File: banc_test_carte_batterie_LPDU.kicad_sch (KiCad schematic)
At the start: 1 part, among them J1 DIN41612_3x32

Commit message: version 26/06/2025 08:31
Signed-off-by: TEST-BANC <TEST-BANC@DOMOMICRON.LOCAL>
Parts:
- added J14, J15, J16, J17, J18, J65, J66, J67: Conn_01x0_P2.54mm_pinheader_vertical, Omiconnecteur:PinHeader_1x01_P2.54mm_V_omi, symbol Omiconnecteur:Conn_01x0_P2.54mm_pinheader_vertical
- added J21, J22, J26: Conn_01x04_P2.54mm_pinheader_vertical, Omiconnecteur:PinHeader_1x04_P2.54mm_V_omi, symbol Omiconnecteur:Conn_01x04_P2.54mm_pinheader_vertical
- added J23, J29: Conn_02x08_Odd_Even, Omiconnecteur:PinHeader_2x08_P2.54mm_V_omi, symbol Omiconnecteur:Conn_02x08_Odd_Even_omi
- added J24, J25: Conn_02x08_Odd_Even, Omiconnecteur:PinHeader_2x02_P2.54mm_V_omi, symbol Omiconnecteur:Conn_02x02_Odd_Even_omi
- added R12, R13, R14, R27, R28, R29, R30, R31, R32, R33, R34, R35: 0, symbol Device:R
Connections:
- net GND: now also J1.B10, J1.B11, J1.B12, J1.B5, J1.B6, J1.B7, J1.B8, J1.B9; no longer J1.B1, J1.B2
- net AI7: now reaches J1.A10
- net AO1: now reaches J1.A11
- net AO2: now reaches J1.A12
- net IN0: now reaches J1.A13
- net IN1: now reaches J1.A14
- net IN2: now reaches J1.A15
- net IN3: now reaches J1.A16
- net IN4: now reaches J1.A17
- net IN5: now reaches J1.A18
- net IN6: now reaches J1.A19
- net at J1.A2: now also J67.1 (Pin_1)
- net IN7: now reaches J1.A20
- net at J1.A21: now also J29.2 (Pin_2)
- net at J1.A22: now also J29.4 (Pin_4)
- net at J1.A23: now also J29.6 (Pin_6)
- net at J1.A24: now also J29.8 (Pin_8)
- net at J1.A25: now also J29.10 (Pin_10)
- net at J1.A26: now also J29.12 (Pin_12)
- net at J1.A27: now also J29.14 (Pin_14)
- net at J1.A28: now also J29.16 (Pin_16)
- net at J1.A29: now also J21.1 (Pin_1), R32.1
- net SORTIE_MULTIPLEXEUR: now reaches J1.A3
- net at J1.A30: now also J21.2 (Pin_2), R33.1
- net at J1.A31: now also J21.3 (Pin_3), R34.1
- net at J1.A32: now also J21.4 (Pin_4), R35.1
- net AI1: now reaches J1.A4
- net AI2: now reaches J1.A5
- net AI3: now reaches J1.A6
- net AI4: now reaches J1.A7
- net AI5: now reaches J1.A8
- net AI6: now reaches J1.A9
- net GND_MCP: now reaches J1.B13
- net GND_MCP: now also J1.B14, J1.B15, J1.B16, J1.B17, J1.B18, J1.B19, J1.B20
- net GND_IO_Ana: now reaches J1.B21
- net GND_IO_Ana: now also J1.B22, J1.B23, J1.B24, J1.B25, J1.B26, J1.B27, J1.B28
- net at J1.B29: now also J26.1 (Pin_1), R28.1
- net at J1.B30: now also J26.2 (Pin_2), R29.1
- net at J1.B31: now also J26.3 (Pin_3), R30.1
- net at J1.B32: now also J26.4 (Pin_4), R31.1
- net at J1.C1: now also J65.1 (Pin_1)
- net at J1.C10: now also J23.16 (Pin_16)
- net at J1.C11: now also J14.1 (Pin_1)
- net at J1.C12: now also J15.1 (Pin_1)
- net S1: now reaches J1.C13
- net S2: now reaches J1.C14
- net S3: now reaches J1.C15
- net S4: now reaches J1.C16
- net S5: now reaches J1.C17
- net S6: now reaches J1.C18
- net S7: now reaches J1.C19
- net S7: now also J1.C20
- net at J1.C2: now also J66.1 (Pin_1)
- net COMMOUT: now reaches J1.C21
- net at J1.C22: now also J24.2 (Pin_2)
- net at J1.C23: now also J24.4 (Pin_4)
- net at J1.C24: now also J25.2 (Pin_2)
- net at J1.C25: now also J25.4 (Pin_4)
- net at J1.C26: now also J18.1 (Pin_1)
- net at J1.C27: now also J16.1 (Pin_1)
- net at J1.C28: now also J17.1 (Pin_1)
- net at J1.C29: now also J22.1 (Pin_1), R12.1
- net at J1.C3: now also J23.2 (Pin_2)
- net at J1.C30: now also J22.2 (Pin_2), R13.1
- net at J1.C31: now also J22.3 (Pin_3), R14.1
- net at J1.C32: now also J22.4 (Pin_4), R27.1
- net at J1.C4: now also J23.4 (Pin_4)
- net at J1.C5: now also J23.6 (Pin_6)
- net at J1.C6: now also J23.8 (Pin_8)
- net at J1.C7: now also J23.10 (Pin_10)
- net at J1.C8: now also J23.12 (Pin_12)
- net at J1.C9: now also J23.14 (Pin_14)
- new net +5V_PIC: R28.2
- new net CLK: J25.1 (Pin_1)
- new net GND_ALIM: J1.B1, J1.B2
- new net GND_TS3A: R12.2, R13.2, R14.2, R27.2
- new net I0: J23.1 (Pin_1)
- new net I1: J23.3 (Pin_3)
- new net I2: J23.5 (Pin_5)
- new net I3: J23.7 (Pin_7)
- new net I4: J23.9 (Pin_9)
- new net I5: J23.11 (Pin_11)
- new net I6: J23.13 (Pin_13)
- new net I7: J23.15 (Pin_15)
- new net IO0: J29.1 (Pin_1)
- new net IO1: J29.3 (Pin_3)
- new net IO2: J29.5 (Pin_5)
- new net IO3: J29.7 (Pin_7)
- new net IO4: J29.9 (Pin_9)
- new net IO5: J29.11 (Pin_11)
- new net IO6: J29.13 (Pin_13)
- new net IO7: J29.15 (Pin_15)
- new net PS13: R29.2
- new net PS14: R30.2
- new net PS15: R31.2
- new net Prog_+5V_PIC: R32.2
- new net Prog_PS13: R33.2
- new net Prog_PS14: R34.2
- new net Prog_PS15: R35.2
- new net Rx: J24.3 (Pin_3)
- new net SDA: J25.3 (Pin_3)
- new net Tx: J24.1 (Pin_1)
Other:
- added sheet MCP23017 (MCP23017.kicad_sch)
- added sheet Relais (Relais.kicad_sch)
- added sheet Support pile (Pile.kicad_sch)
- note added: "permetre de connceter une carte relais de 4 si on soude pas la resistance 0 ohm"
- moved on the sheet: J1

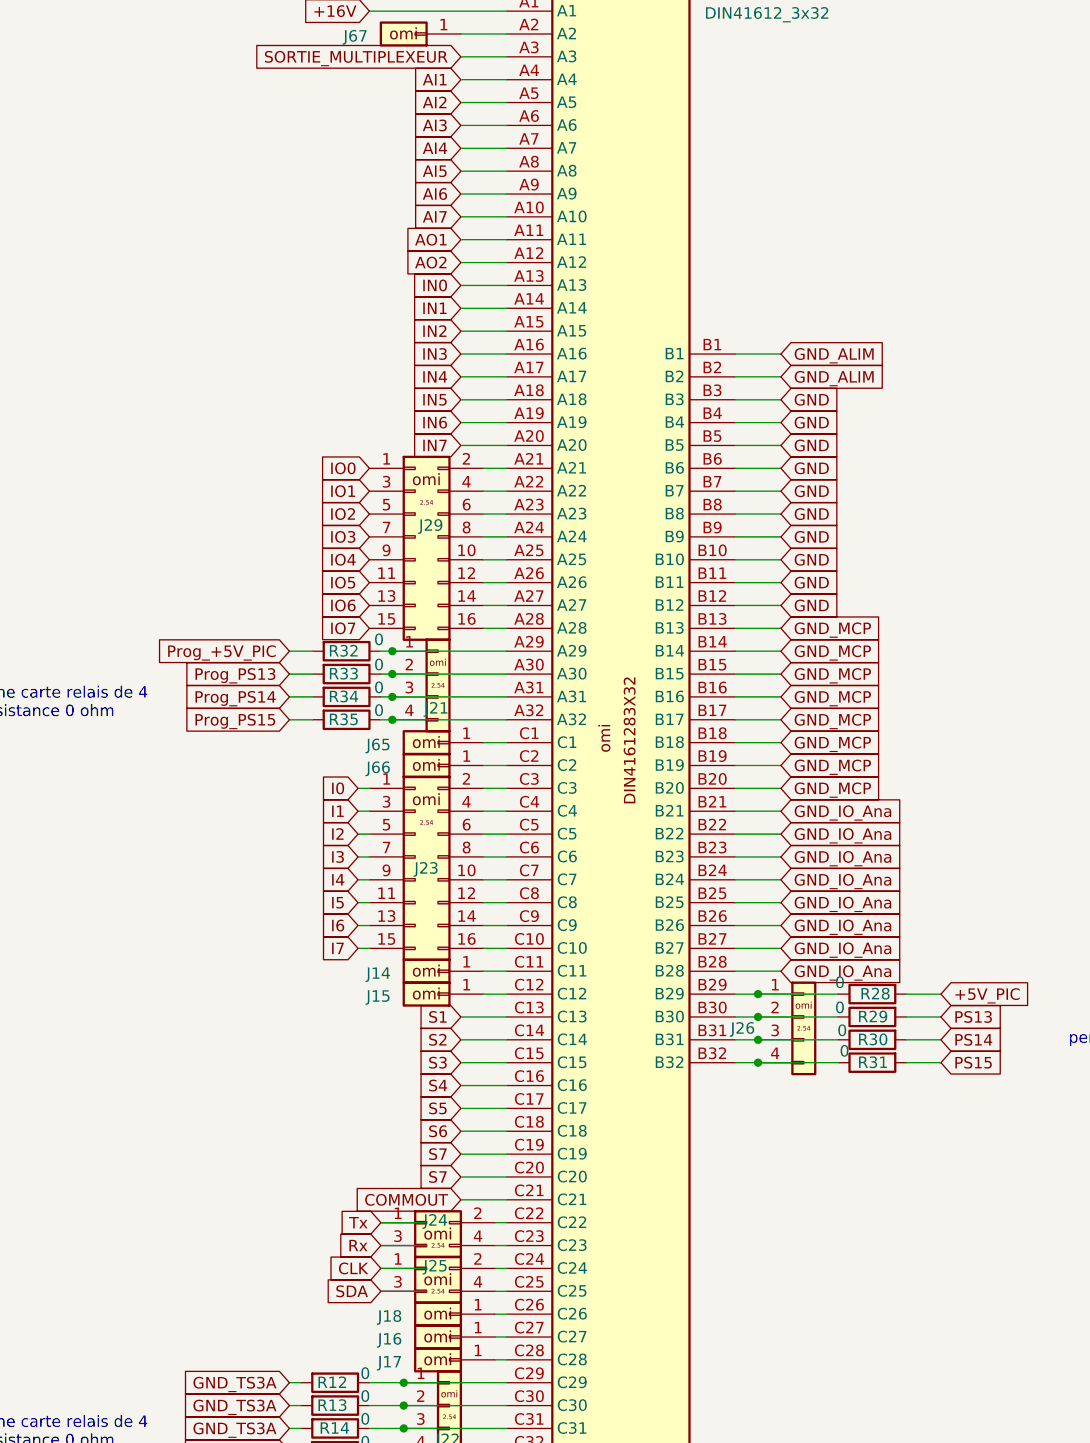
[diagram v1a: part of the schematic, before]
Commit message: 26/06/2025  11:50 Signed-off-by: TEST-BANC <TEST-BANC@DOMOMICRON.LOCAL>
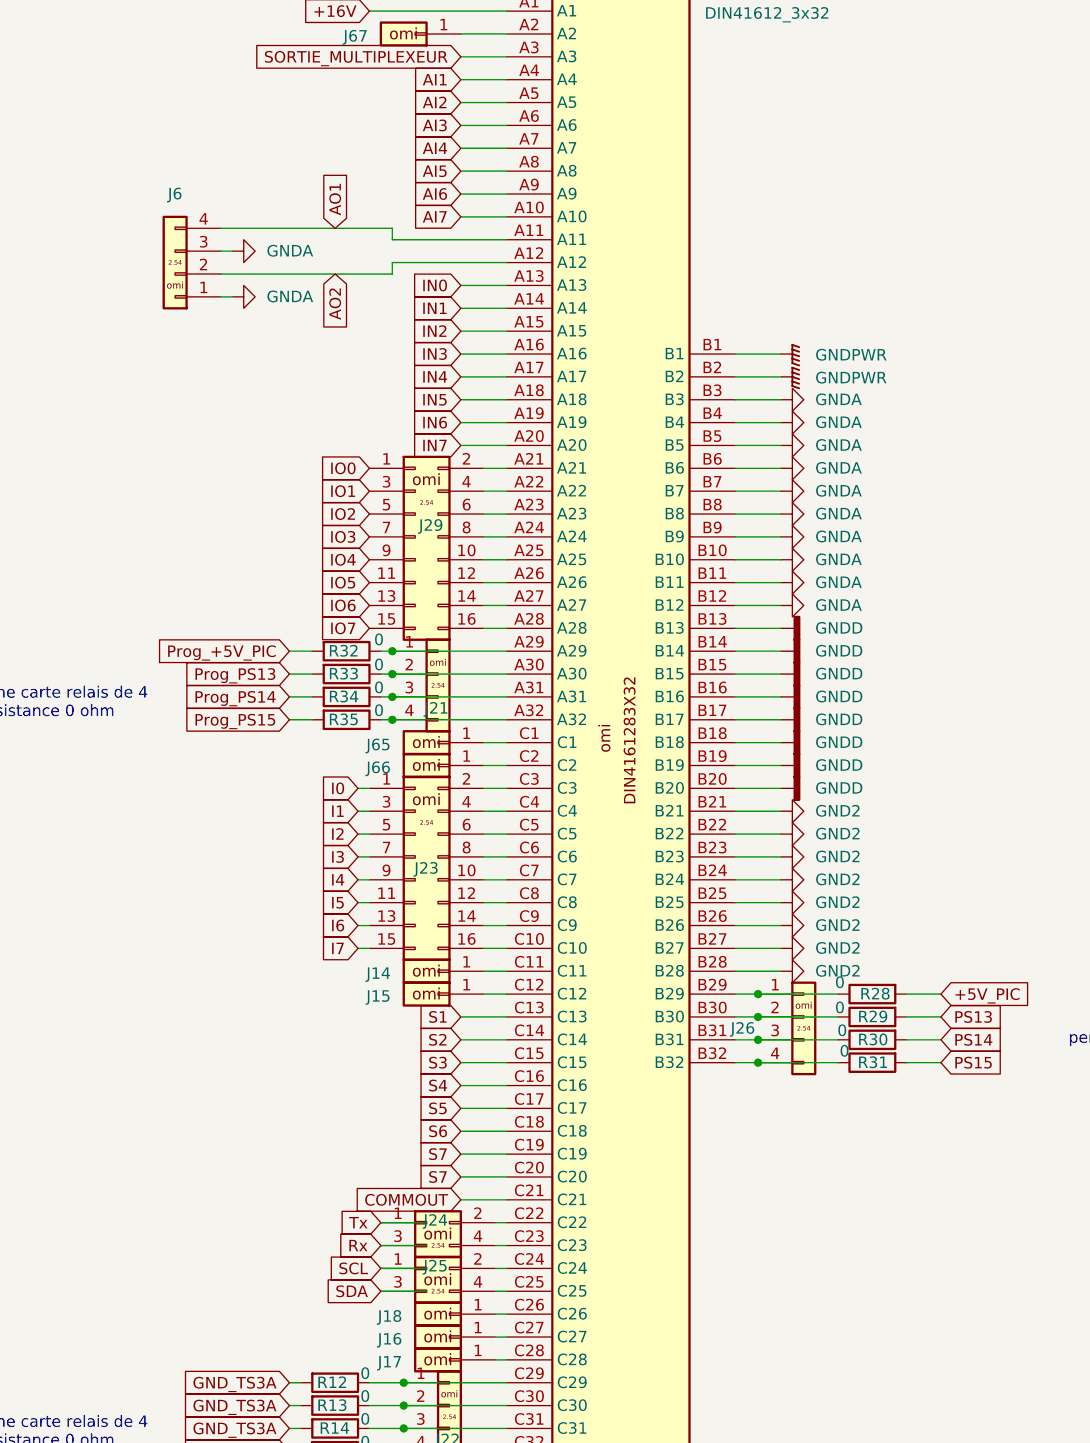
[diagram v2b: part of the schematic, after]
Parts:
- added J6: Conn_01x04_P2.54mm_pinheader_vertical, Omiconnecteur:PinHeader_1x04_P2.54mm_V_omi, symbol Omiconnecteur:Conn_01x04_P2.54mm_pinheader_vertical
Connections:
- net AO1: now also J6.4 (Pin_4)
- net AO2: now also J6.2 (Pin_2)
- net GND: no longer J1.B10, J1.B11, J1.B12, J1.B3, J1.B4, J1.B5, J1.B6, J1.B7, J1.B8, J1.B9
- net CLK renamed SCL
- net GND_ALIM renamed GNDPWR
- net GND_IO_Ana renamed GND2
- net GND_MCP renamed GNDD
- new net GNDA: J1.B10, J1.B11, J1.B12, J1.B3, J1.B4, J1.B5, J1.B6, J1.B7, J1.B8, J1.B9, J6.1 (Pin_1), J6.3 (Pin_3)
